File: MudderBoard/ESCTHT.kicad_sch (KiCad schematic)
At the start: 82 parts, among them M3 N-MOSFET, M4 N-MOSFET, U8 LM5122QMH/NOPB, U9 LM5122QMH/NOPB

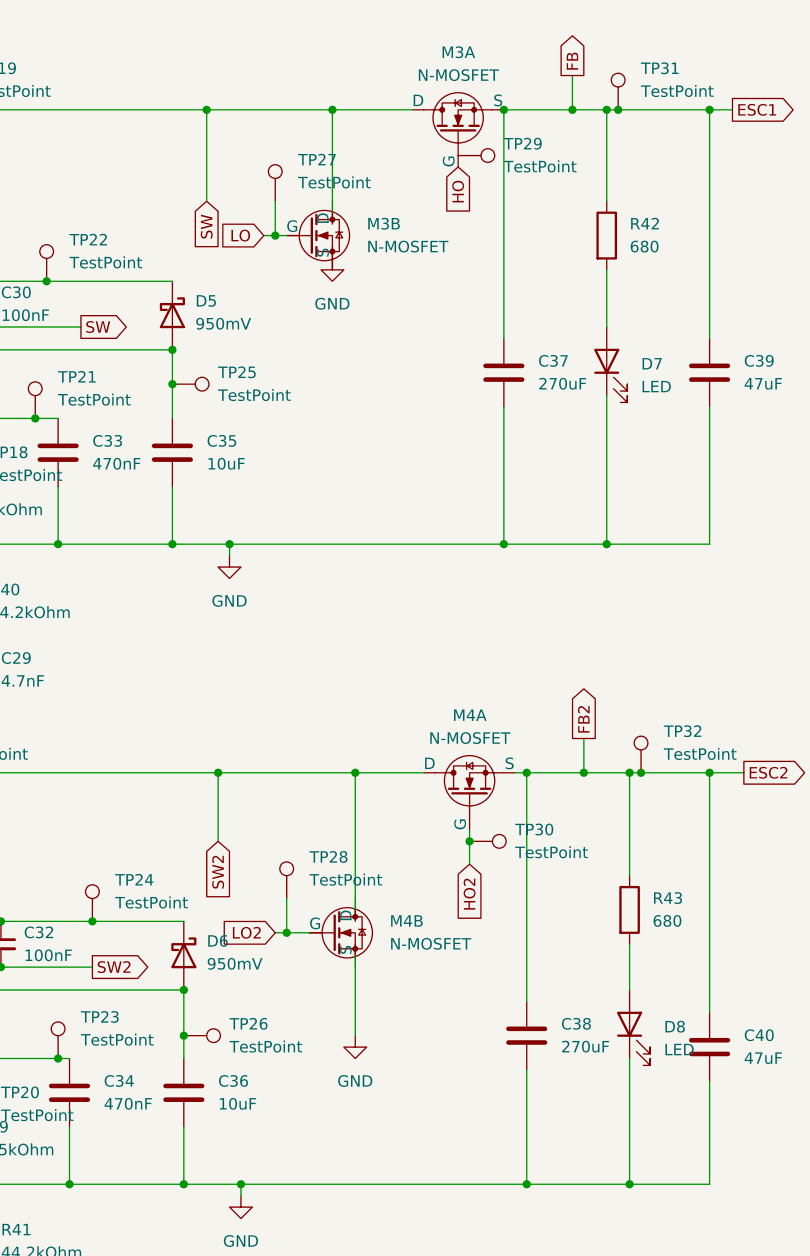
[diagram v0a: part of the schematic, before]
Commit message: Layout
ESC
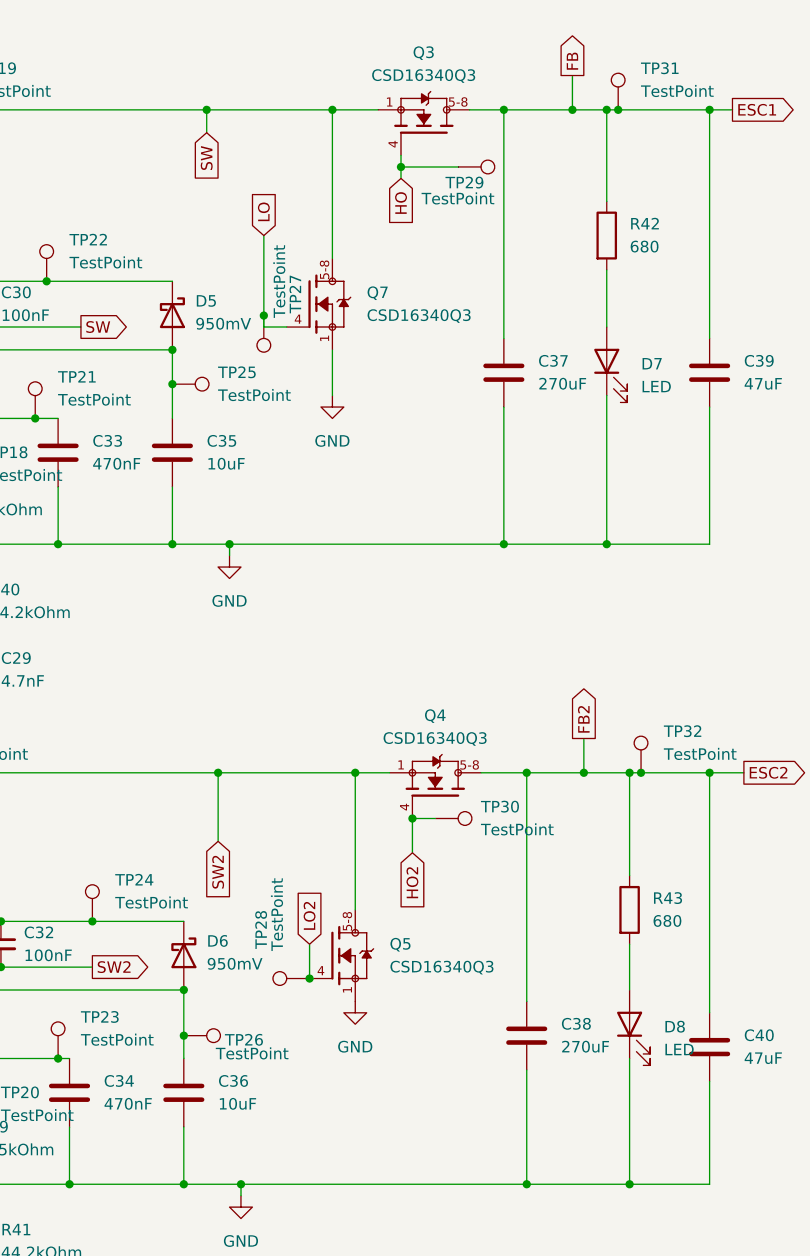
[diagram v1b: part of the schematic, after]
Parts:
- removed M3, M4: N-MOSFET, Lidar_Foot:TRANS_CSD17308Q3, symbol DI110N04PQ-AQ:nMOS
- added Q3, Q4, Q5, Q7: CSD16340Q3, ColinFET1:TRANS_CSD16340Q3, symbol ColinFET1:CSD16340Q3
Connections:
- net ESC1: now also Q3.5-8
- net ESC2: now also Q4.5-8
- net GND: now also Q5.1, Q7.1
- net HO: now also TP29.1, Q3.4
- net HO2: now also Q4.4
- net LO: now also Q7.4
- net LO2: now also Q5.4
- net SW: now also Q3.1, Q7.5-8
- net SW2: now also Q4.1, Q5.5-8
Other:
- moved on the sheet: TP27, TP29, TP30
